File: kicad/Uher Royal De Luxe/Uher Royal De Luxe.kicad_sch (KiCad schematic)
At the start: 6 parts

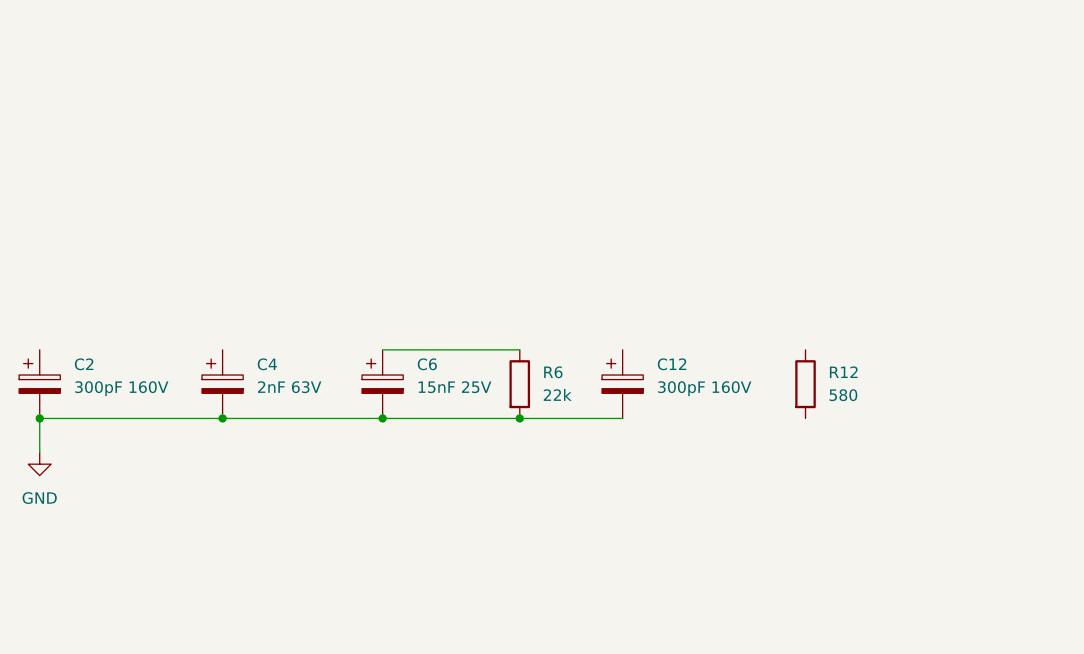
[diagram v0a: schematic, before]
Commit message: Added Documents and Progress
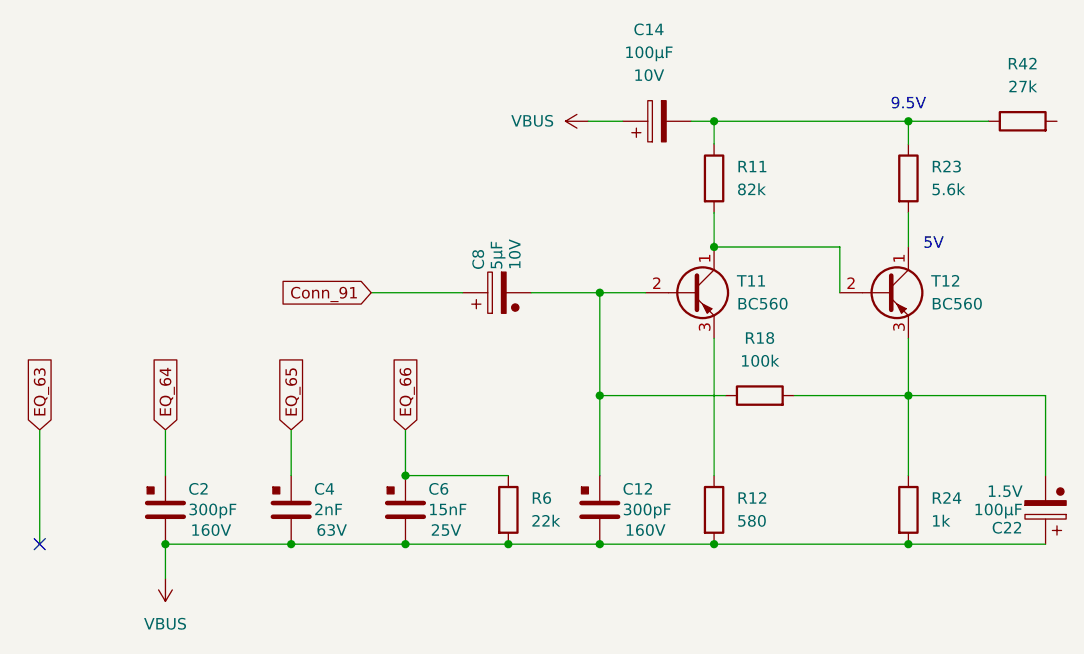
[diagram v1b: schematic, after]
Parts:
- removed C12, C2: 300pF 160V, symbol Device:C_Polarized
- removed C4: 2nF 63V, symbol Device:C_Polarized
- removed C6: 15nF 25V, symbol Device:C_Polarized
- added C12, C2: 300pF, symbol Uher_Symbols:C_Styroflex
- added C14: 100µF, symbol Uher_Symbols:C_Polarized_Electrolytic
- added C22: 100µF, symbol Uher_Symbols:C_Polarized_Tantalum
- added C4: 2nF, symbol Uher_Symbols:C_Styroflex
- added C6: 15nF, symbol Uher_Symbols:C_Styroflex
- added C8: 5µF, symbol Uher_Symbols:C_Polarized_Tantalum
- added R11: 82k, symbol Device:R
- added R18: 100k, symbol Device:R
- added R23: 5.6k, symbol Device:R
- added R24: 1k, symbol Device:R
- added R42: 27k, symbol Device:R
- added T11, T12: BC560, Package_TO_SOT_THT:TO-92_Inline, symbol Transistor_BJT:BC560
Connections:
- net GND is gone; now on net VBUS: R6.2
- net EQ_66: now reaches R6.1
- net EQ_66: now also C6.1
- net at R12.1: now also T11.3 (E)
- net VBUS: now reaches R12.2
- net VBUS: now also C12.2, C14.1, C2.2, C22.1, C4.2, C6.2, R24.2
- new net: C14.2, R11.1, R23.1, R42.1
- new net: R23.2, T12.1 (C)
- new net: R11.2, T11.1 (C), T12.2 (B)
- new net: C12.1, C8.2, R18.1, T11.2 (B)
- new net: C22.2, R18.2, R24.1, T12.3 (E)
- new net Conn_91: C8.1
- new net EQ_64: C2.1
- new net EQ_65: C4.1
- no-connect marks 0 -> 1
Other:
- note added: "5V"
- note added: "9.5V"
- moved on the sheet: R12, R6
